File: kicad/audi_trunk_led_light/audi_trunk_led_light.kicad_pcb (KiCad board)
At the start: 2 copper layers, 96.1 x 42.2 mm, 77 parts, among them P1 CONN_01X02, P2 CONN_01X02

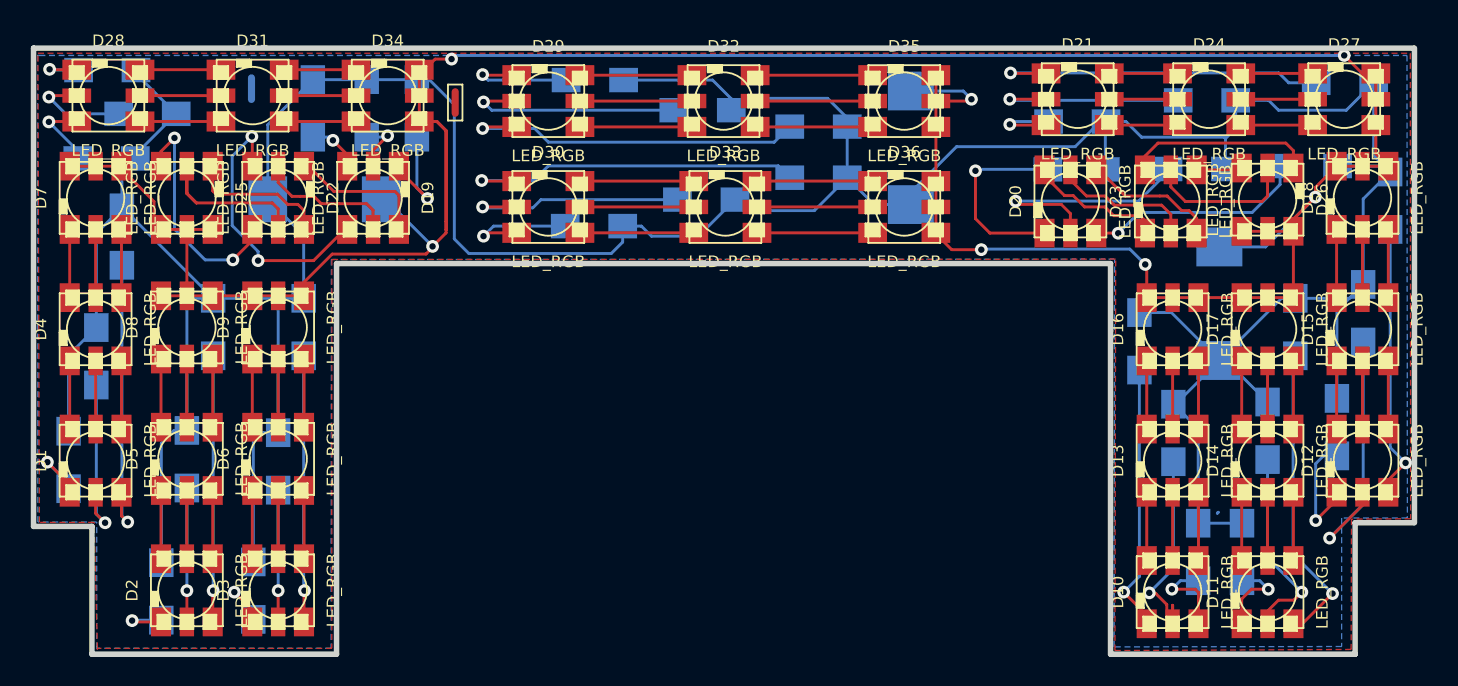
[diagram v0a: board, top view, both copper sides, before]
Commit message: clean up
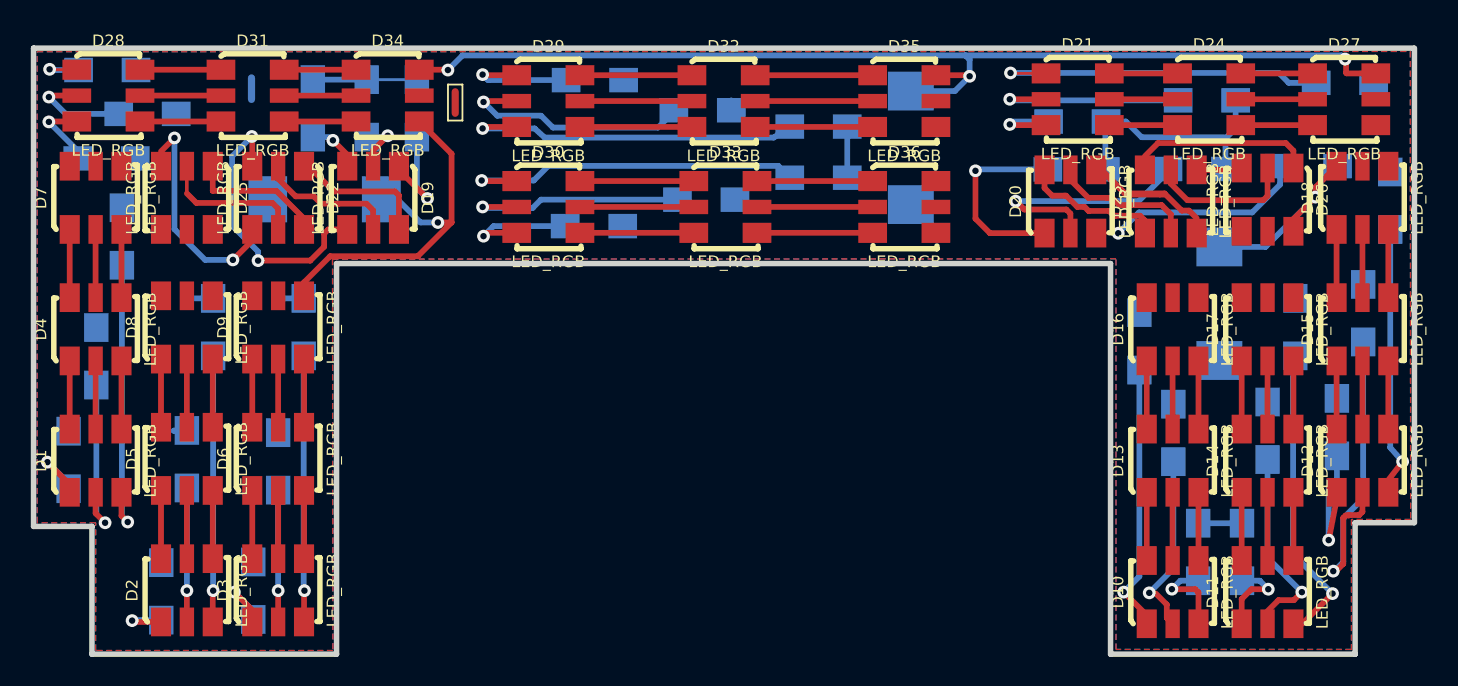
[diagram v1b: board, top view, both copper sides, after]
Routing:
- net Net-(P1-Pad1): track 297.5 -> 44.4 mm
- net Net-(D16-PadBC): track 215.2 -> 123.1 mm, vias 7 -> 5
- net Net-(D20-PadBC): track 9.41 -> 16.5 mm
- net Net-(D12-PadGA): track 18.7 -> 24.7 mm
- net Net-(D20-PadRC): track 10.5 -> 13.2 mm
- net Net-(D10-PadGA): track 15.5 -> 12.9 mm
- net Net-(D20-PadGA): track 17.2 -> 18.5 mm
- net Net-(D20-PadGC): track 9.99 -> 11.3 mm
- net Net-(D12-PadRA): track 8.23 -> 9.48 mm
- net Net-(D29-PadGA): track 15.8 -> 16.9 mm
- net Net-(D19-PadBC): track 19.7 -> 20.4 mm
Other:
- net class Default: trace_width 0.2032 -> 0.4
